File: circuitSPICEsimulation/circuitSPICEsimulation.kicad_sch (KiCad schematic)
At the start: 20 parts, among them U1 Opamp_Dual, U2 Opamp_Dual, U3 Opamp_Dual, U4 Opamp_Dual, U5 Opamp_Dual

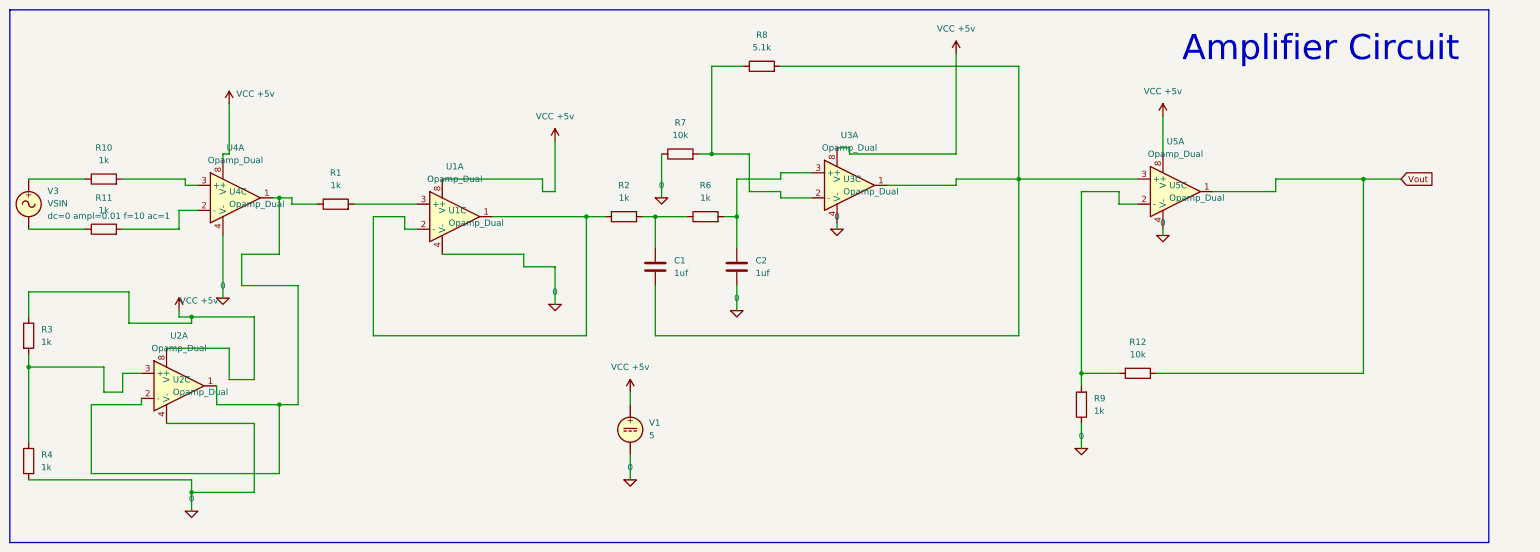
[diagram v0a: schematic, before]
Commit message: Getting the simulation to work
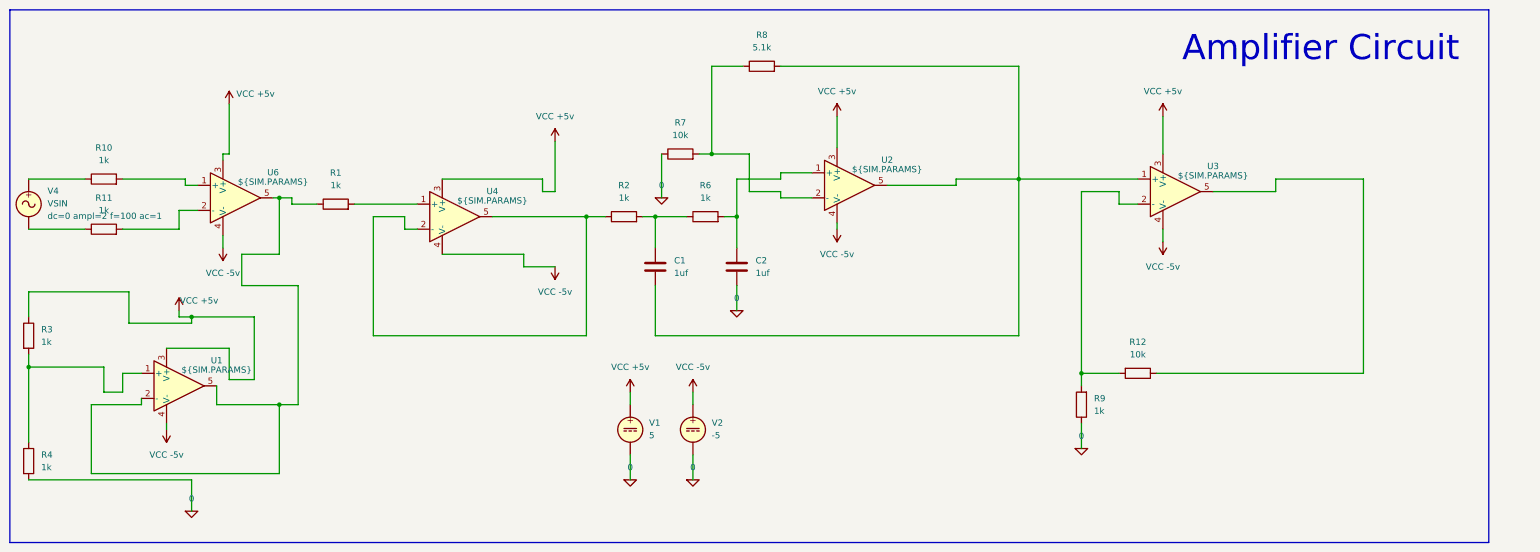
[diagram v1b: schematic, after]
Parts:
- removed U1, U2, U3, U4, U5: Opamp_Dual, symbol Device:Opamp_Dual
- removed V3: VSIN, symbol Simulation_SPICE:VSIN
- added U1, U2, U3, U4, U6: ${SIM.PARAMS}, symbol Simulation_SPICE:OPAMP
- added V2: -5, symbol Simulation_SPICE:VDC
- added V4: VSIN, symbol Simulation_SPICE:VSIN
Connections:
- net 0: now also V2.2
- net VCC +5v: now also U1.3 (V+), U2.3 (V+), U3.3 (V+), U4.3 (V+), U6.3 (V+)
- net at R1.1: now also U1.2 (-), U1.5, U6.5
- net at R3.2, R4.1: now also U1.1 (+)
- net at C2.1, R6.2: now also U2.1 (+)
- net at R11.2: now also U6.2 (-)
- net at R10.2: now also U6.1 (+)
- net at R7.2, R8.1: now also U2.2 (-)
- net at C1.2, R8.2: now also U2.5, U3.1 (+)
- net at R12.2, R9.2: now also U3.2 (-)
- net at R2.1: now also U4.2 (-), U4.5
- net at R1.2: now also U4.1 (+)
- net at R10.1: now also V4.1
- net at R11.1: now also V4.2
- net Vout: no longer names the net of R12.1
- net Vout: now also U3.5
- new net VCC -5v: U1.4 (V-), U2.4 (V-), U3.4 (V-), U4.4 (V-), U6.4 (V-), V2.1
